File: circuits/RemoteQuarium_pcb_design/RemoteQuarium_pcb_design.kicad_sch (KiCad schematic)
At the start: 33 parts, among them J1 Power_terminal, J10 LCD_pins, J11 Feeder_servo_pins, J12 ESP_pins, J13 PH_sensor_sockets, J14 Ph_sesnor-pins, J15 Power & D3-D4, J16 Reset_button_terminal, J2 ESP left side sockets, J3 ESP right side sockets, J4 Relay_terminal, J5 SREG_pins, J6 Temp_sensor_terminal, J7 Water_sensor_terminal, J8 Light_sensor_terminal, J9 MUX_pins, Q1 BC547, U2 74HC595, U3 CD4052B

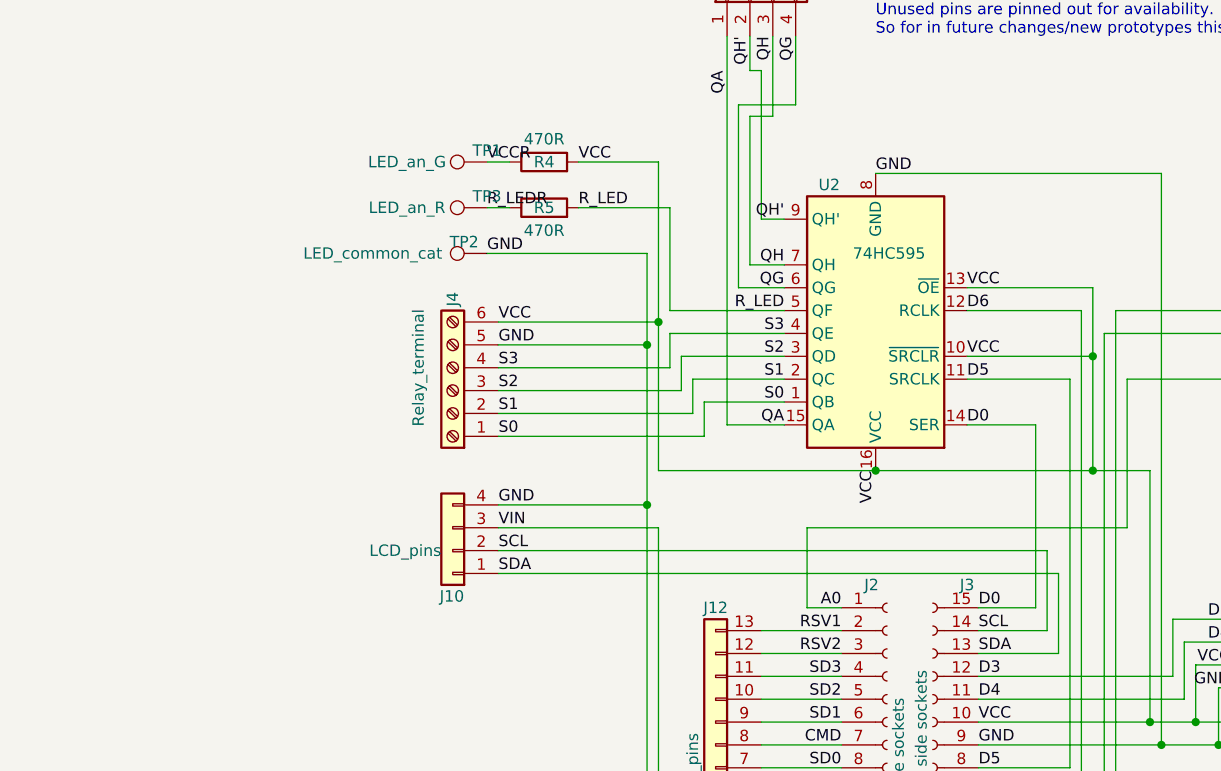
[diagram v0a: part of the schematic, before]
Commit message: Added more complex logging and notification testing should work, app builds and is usable, but need to add react SVG libs for the charts to workgit add .
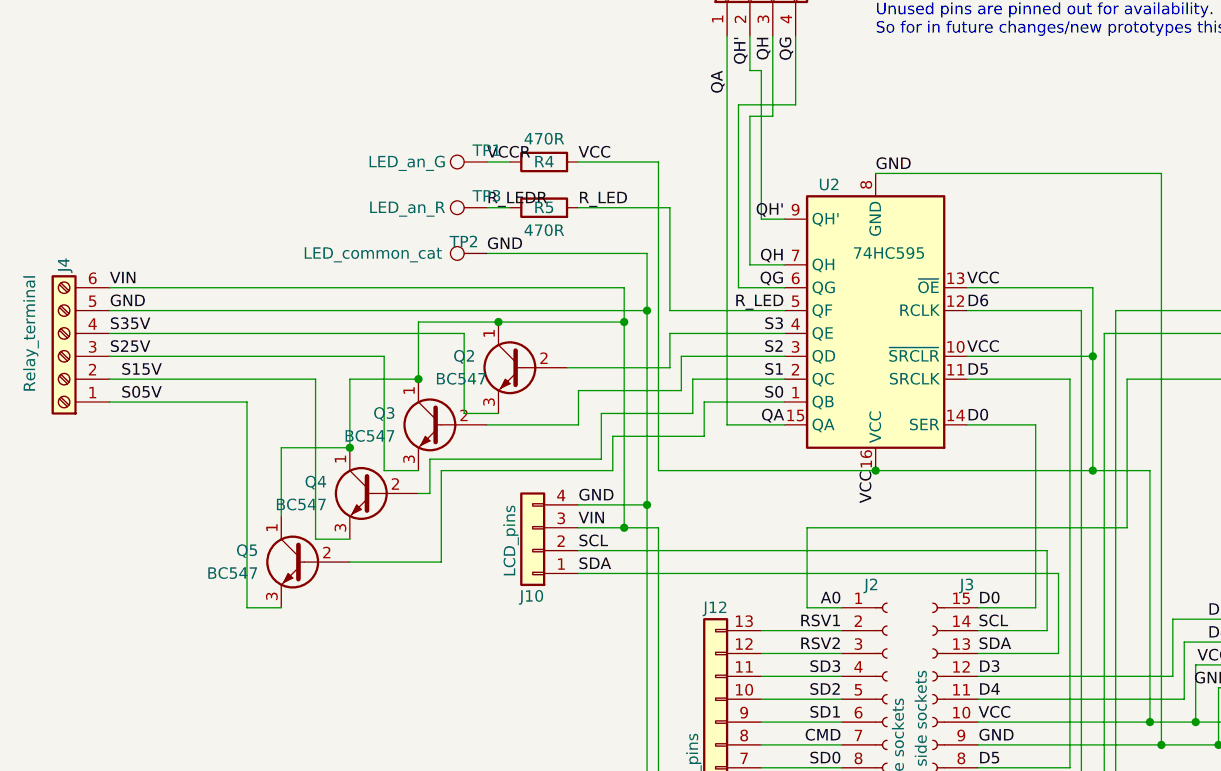
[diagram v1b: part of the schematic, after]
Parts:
- added Q2, Q3, Q4, Q5: BC547, Package_TO_SOT_THT:TO-92_Inline, symbol Transistor_BJT:BC547
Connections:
- net S0: now also Q5.2 (B); no longer J4.1 (Pin_1)
- net S1: now also Q4.2 (B); no longer J4.2 (Pin_2)
- net S2: now also Q3.2 (B); no longer J4.3 (Pin_3)
- net S3: now also Q2.2 (B); no longer J4.4 (Pin_4)
- net VCC: no longer J4.6 (Pin_6)
- net VIN: now also J4.6 (Pin_6), Q2.1 (C), Q3.1 (C), Q4.1 (C), Q5.1 (C)
- new net S05V: J4.1 (Pin_1), Q5.3 (E)
- new net S15V: J4.2 (Pin_2), Q4.3 (E)
- new net S25V: J4.3 (Pin_3), Q3.3 (E)
- new net S35V: J4.4 (Pin_4), Q2.3 (E)
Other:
- moved on the sheet: J10, J4
